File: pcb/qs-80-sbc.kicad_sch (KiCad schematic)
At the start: 57 parts, among them J1 BUS, J2 USB_B, J3 DE9_Socket, J4 Atmel-JTAG-10, J5 KEYBOARD, J6 MOUSE, SW1 ON, SW2 RESET, SW3 NMI, U1 Z84C0020, U2 CY62256-70PC, U22 MAX232, U3 ATmega328P-P, U4 SST39SF010, U5 ATF1504AS-xJx44, U6 TL16C2550PFBR, U7 74HC273, U8 VERA MJ, U9 74HC138, Y1 14.7456 MHz, Y2 16MHz

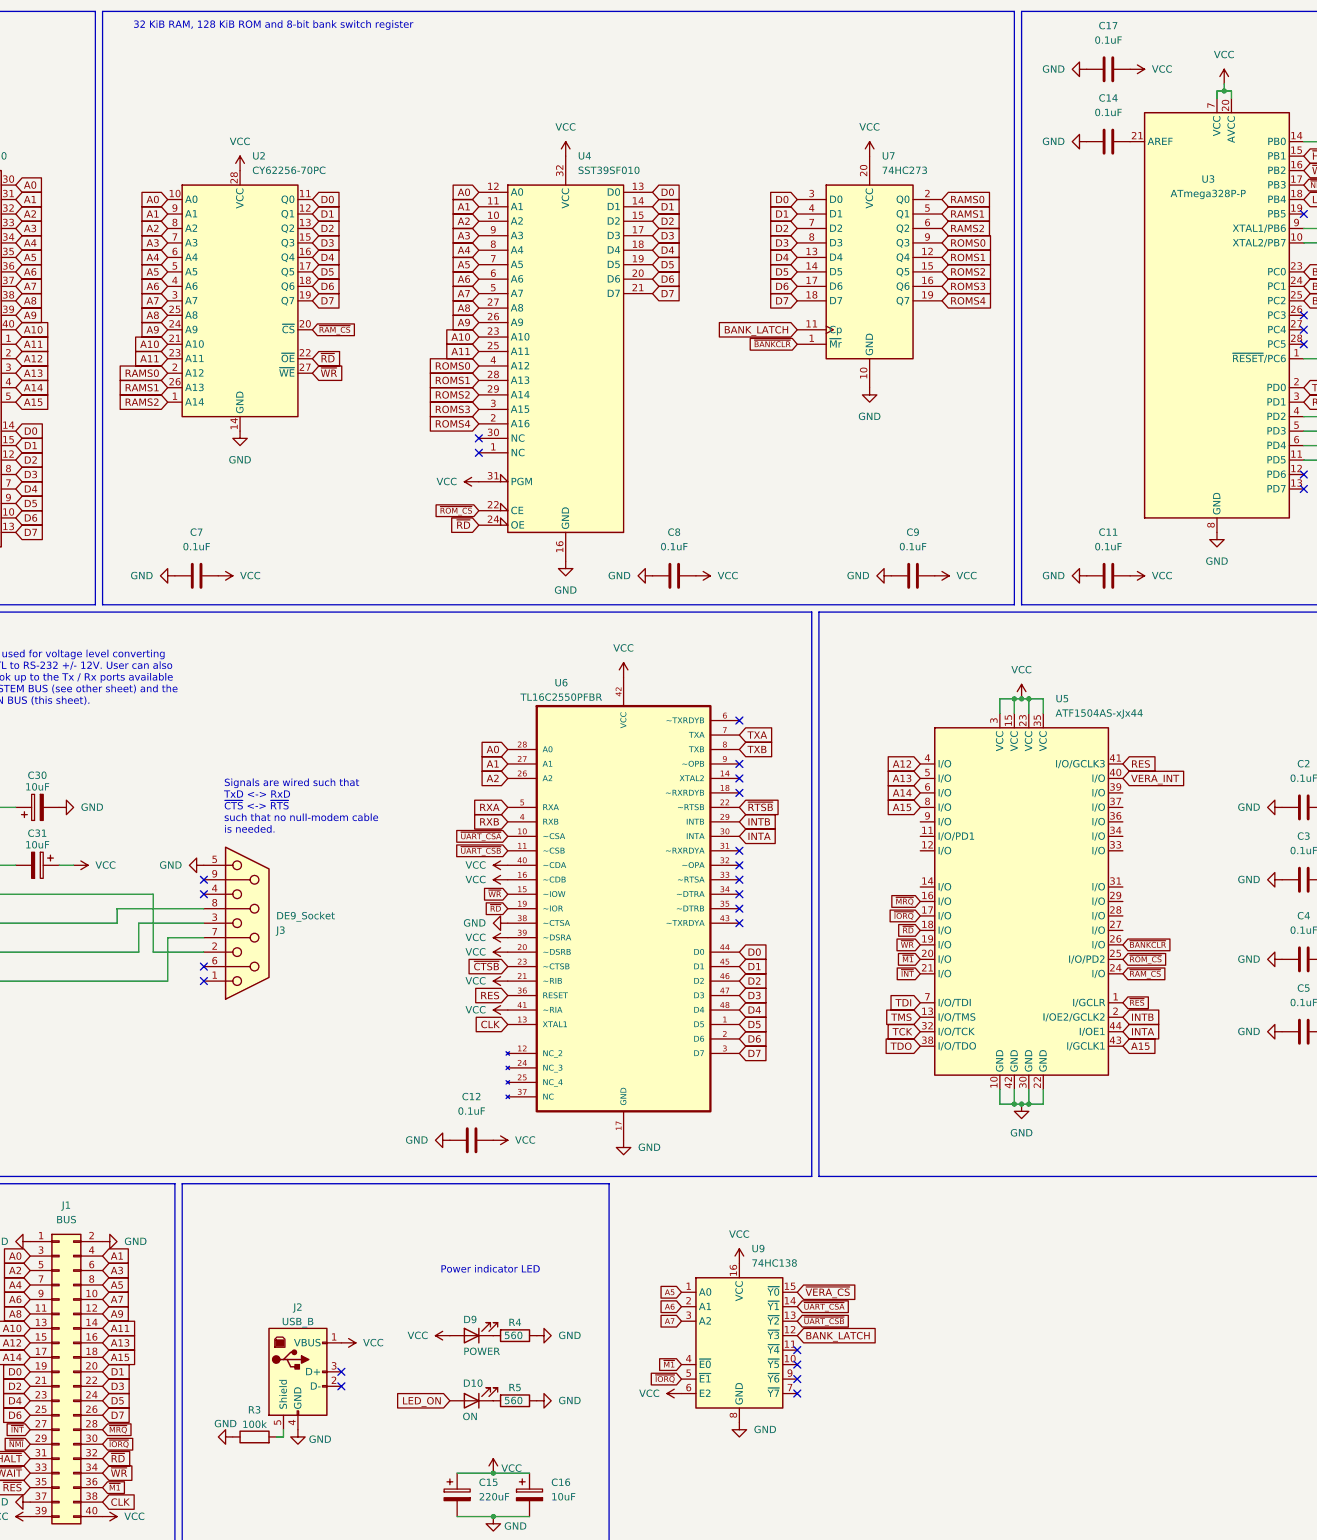
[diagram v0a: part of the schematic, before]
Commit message: Tuning I/O ports
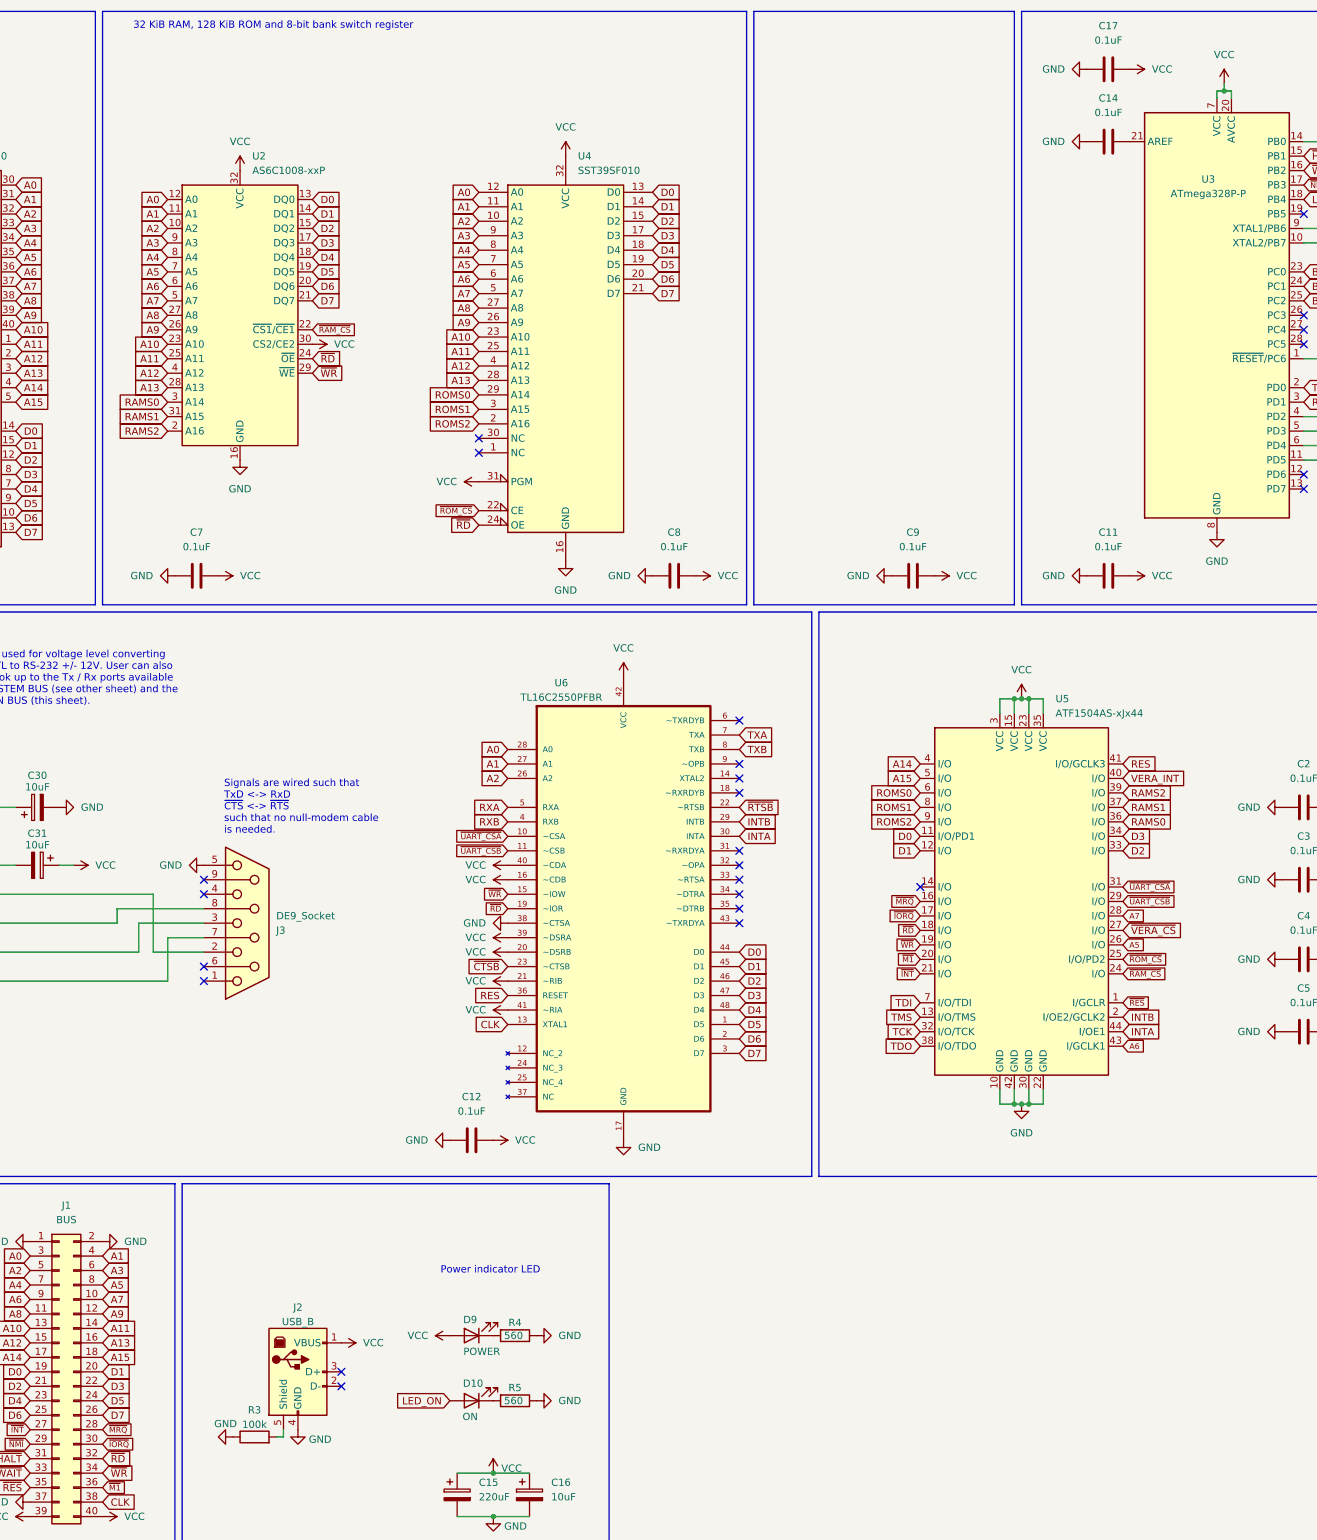
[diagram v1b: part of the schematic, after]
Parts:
- removed U2: CY62256-70PC, Package_DIP:DIP-28_W15.24mm, symbol Memory_RAM:CY62256-70PC
- removed U7: 74HC273, Package_DIP:DIP-20_W7.62mm_Socket, symbol 74xx:74HC273
- removed U9: 74HC138, symbol 74xx:74HC138
- added U2: AS6C1008-xxP, Package_DIP:DIP-32_W15.24mm, symbol Memory_RAM:AS6C1008-xxP
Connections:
- net ROMS3 is gone; now on net ROMS1: U4.3 (A15)
- net ROMS4 is gone; now on net ROMS2: U4.2 (A16)
- net ~{BANKCLR} is gone; now on net A5: U5.26 (I/O)
- net A0: now also U2.12 (A0)
- net A1: now also U2.11 (A1)
- net A10: now also U2.23 (A10)
- net A11: now also U2.25 (A11)
- net A12: now also U4.4 (A12), U2.4 (A12); no longer U5.4 (I/O)
- net A13: now also U4.28 (A13), U2.28 (A13); no longer U5.5 (I/O)
- net A14: now also U5.4 (I/O); no longer U5.6 (I/O)
- net A15: now also U5.5 (I/O); no longer U5.43 (I/GCLK1), U5.8 (I/O)
- net A2: now also U2.10 (A2)
- net A3: now also U2.9 (A3)
- net A4: now also U2.8 (A4)
- net A5: now also U2.7 (A5)
- net A6: now also U5.43 (I/GCLK1), U2.6 (A6)
- net A7: now also U5.28 (I/O), U2.5 (A7)
- net A8: now also U2.27 (A8)
- net A9: now also U2.26 (A9)
- net D0: now also U5.11 (I/O/PD1), U2.13 (DQ0)
- net D1: now also U5.12 (I/O), U2.14 (DQ1)
- net D2: now also U5.33 (I/O), U2.15 (DQ2)
- net D3: now also U5.34 (I/O), U2.17 (DQ3)
- net D4: now also U2.18 (DQ4)
- net D5: now also U2.19 (DQ5)
- net D6: now also U2.20 (DQ6)
- net D7: now also U2.21 (DQ7)
- net GND: now also U2.16 (GND)
- net RAMS0: now also U5.36 (I/O), U2.3 (A14)
- net RAMS1: now also U5.37 (I/O), U2.31 (A15)
- net RAMS2: now also U5.39 (I/O), U2.2 (A16)
- net ROMS0: now also U4.29 (A14), U5.6 (I/O); no longer U4.4 (A12)
- net ROMS1: now also U5.8 (I/O); no longer U4.28 (A13)
- net ROMS2: now also U5.9 (I/O); no longer U4.29 (A14)
- net VCC: now also U2.30 (CS2/CE2), U2.32 (VCC)
- net ~{RAM_CS}: now also U2.22 (~{CS1}/~{CE1})
- net ~{RD}: now also U2.24 (~{OE})
- net ~{UART_CSA}: now also U5.31 (I/O)
- net ~{UART_CSB}: now also U5.29 (I/O)
- net ~{VERA_CS}: now also U5.27 (I/O)
- net ~{WR}: now also U2.29 (~{WE})
- no-connect marks 35 -> 32
